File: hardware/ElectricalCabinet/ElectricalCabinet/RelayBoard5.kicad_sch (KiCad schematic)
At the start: 0 parts

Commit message: Further wiring updates
Populated 6100 Bus
Corrected number of relay boards
Added 110v outputs to relay boards and noted light positon
Uploaded light scheme to documents folder
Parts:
- added C5: 0.1uF, Capacitor_SMD:C_0805_2012Metric, symbol Device:C
- added D33, D34, D35, D36, D37, D38, D39, D40: LED, LED_SMD:LED_0805_2012Metric, symbol Device:LED
- added J10: Screw_Terminal_01x06, TerminalBlock:TerminalBlock_MaiXu_MX126-5.0-06P_1x06_P5.00mm, symbol Connector:Screw_Terminal_01x06
- added J11: Screw_Terminal_01x09, TerminalBlock:TerminalBlock_MaiXu_MX126-5.0-09P_1x09_P5.00mm, symbol Connector:Screw_Terminal_01x09
- added K33, K34, K35, K36, K37, K38, K39, K40: G3MB-202P DC5, TrafficLightLibrary:G3MB_202P_DC5, symbol TrafficLightLibrary:G3MB-202P_DC5
- added R33, R34, R35, R36, R37, R38, R39, R40: 1kΩ, Resistor_SMD:R_0805_2012Metric, symbol Device:R
- added U6: TPIC6B595N, TrafficLightLibrary:TPIC6B595N, symbol TrafficLightLibrary:TPIC6B595N
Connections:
- new net: J11.9 (Pin_9), K33.1, K34.1, K35.1, K36.1, K37.1, K38.1, K39.1, K40.1
- new net: J11.7 (Pin_7), K39.2
- new net: D33.2 (A), D34.2 (A), D35.2 (A), D36.2 (A), D37.2 (A), D38.2 (A), D39.2 (A), D40.2 (A), K33.3, K34.3, K35.3, K36.3, K37.3, K38.3, K39.3, K40.3
- new net: K39.4, R39.2, U6.16 (DRAIN6)
- new net: D39.1 (K), R39.1
- new net: J10.1 (Pin_1), U6.18 (SEROUT)
- new net: C5.1, J10.2 (Pin_2), U6.10 (GND), U6.11 (GND), U6.19 (GND), U6.9 (~{G})
- new net: J10.3 (Pin_3), U6.13 (SRCK)
- new net: J10.4 (Pin_4), U6.12 (RCK)
- new net: C5.2, J10.6 (Pin_6), U6.2 (VCC), U6.8 (~{SRCLR})
- new net: D34.1 (K), R34.1
- new net: D35.1 (K), R35.1
- new net: K34.4, R34.2, U6.5 (DRAIN1)
- new net: D37.1 (K), R37.1
- new net: K37.4, R37.2, U6.14 (DRAIN4)
- new net: J11.6 (Pin_6), K38.2
- new net: K38.4, R38.2, U6.15 (DRAIN5)
- new net: J11.8 (Pin_8), K40.2
- new net: K40.4, R40.2, U6.17 (DRAIN7)
- new net: D38.1 (K), R38.1
- new net: D40.1 (K), R40.1
- new net: D36.1 (K), R36.1
- new net: K33.4, R33.2, U6.4 (DRAIN0)
- new net: K35.4, R35.2, U6.6 (DRAIN2)
- new net: K36.4, R36.2, U6.7 (DRAIN3)
- new net: D33.1 (K), R33.1
- new net: J11.1 (Pin_1), K33.2
- new net: J11.4 (Pin_4), K36.2
- new net: J11.3 (Pin_3), K35.2
- new net: J11.2 (Pin_2), K34.2
- new net: J11.5 (Pin_5), K37.2
- new net SERIN: J10.5 (Pin_5), U6.3 (SERIN)
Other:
- note added: "RELAY MODULE 5"

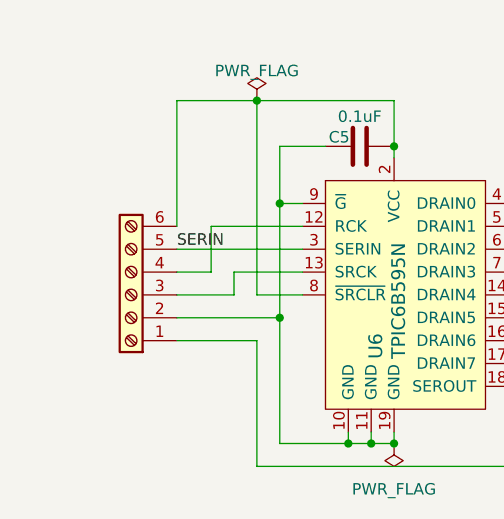
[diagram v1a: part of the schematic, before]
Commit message: Electrical Cabinet done
Electrical Cabinet done, let me know if there are any changes or mistakes.
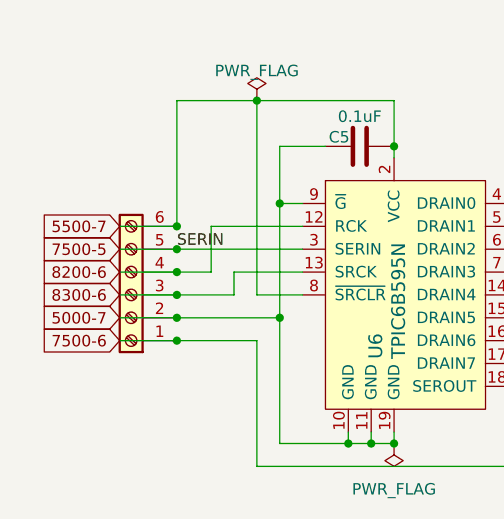
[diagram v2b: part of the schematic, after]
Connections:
- net 7500-6: now reaches J10.1 (Pin_1), U6.18 (SEROUT)
- net 5000-7: now reaches C5.1, J10.2 (Pin_2), U6.10 (GND), U6.11 (GND), U6.19 (GND), U6.9 (~{G})
- net 8300-6: now reaches J10.3 (Pin_3), U6.13 (SRCK)
- net 8200-6: now reaches J10.4 (Pin_4), U6.12 (RCK)
- net 5500-7: now reaches C5.2, J10.6 (Pin_6), U6.2 (VCC), U6.8 (~{SRCLR})
- net SERIN renamed 7500-5
